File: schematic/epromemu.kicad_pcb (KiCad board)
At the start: 2 copper layers, 6 parts, among them J1 EPROM Connector, U1 Teensy4.1, U2 TXS0108EPW, U3 TXS0108EPW, U4 TXS0108EPW, U5 TXS0108EPW

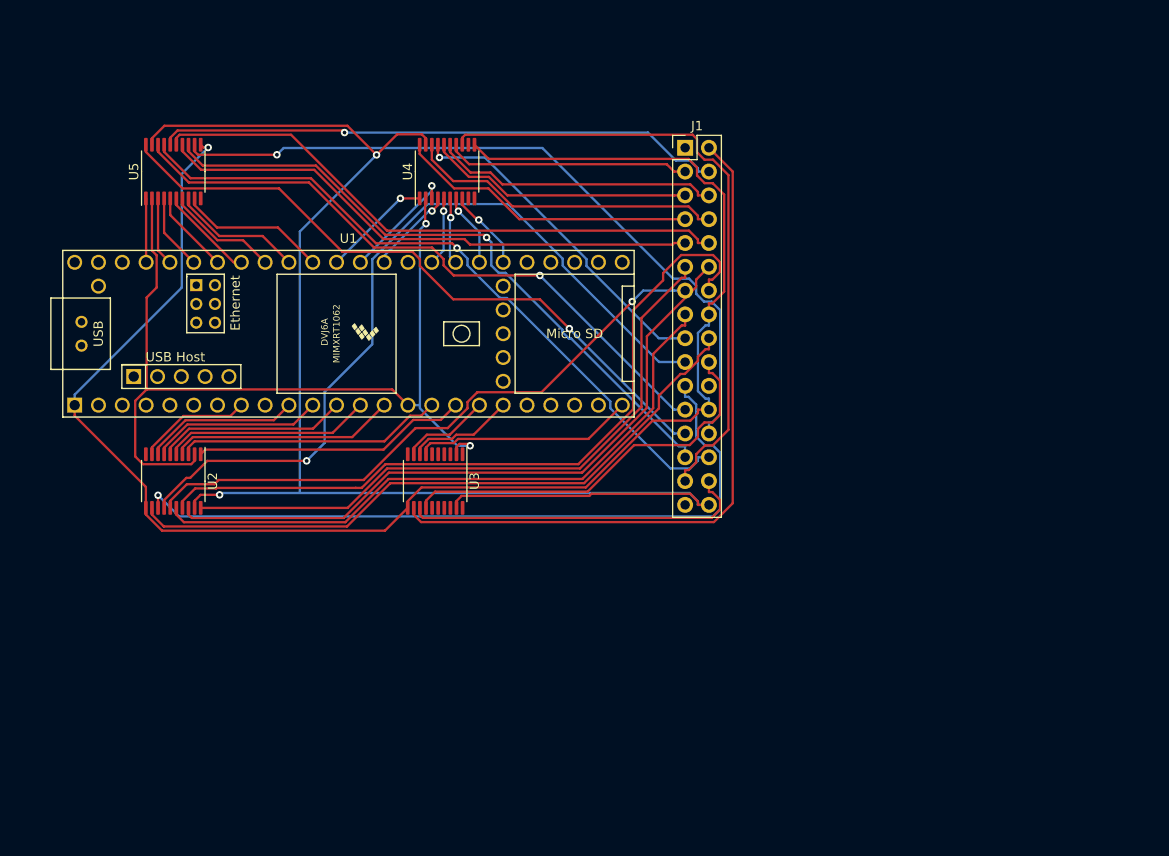
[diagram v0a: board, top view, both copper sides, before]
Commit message: updates
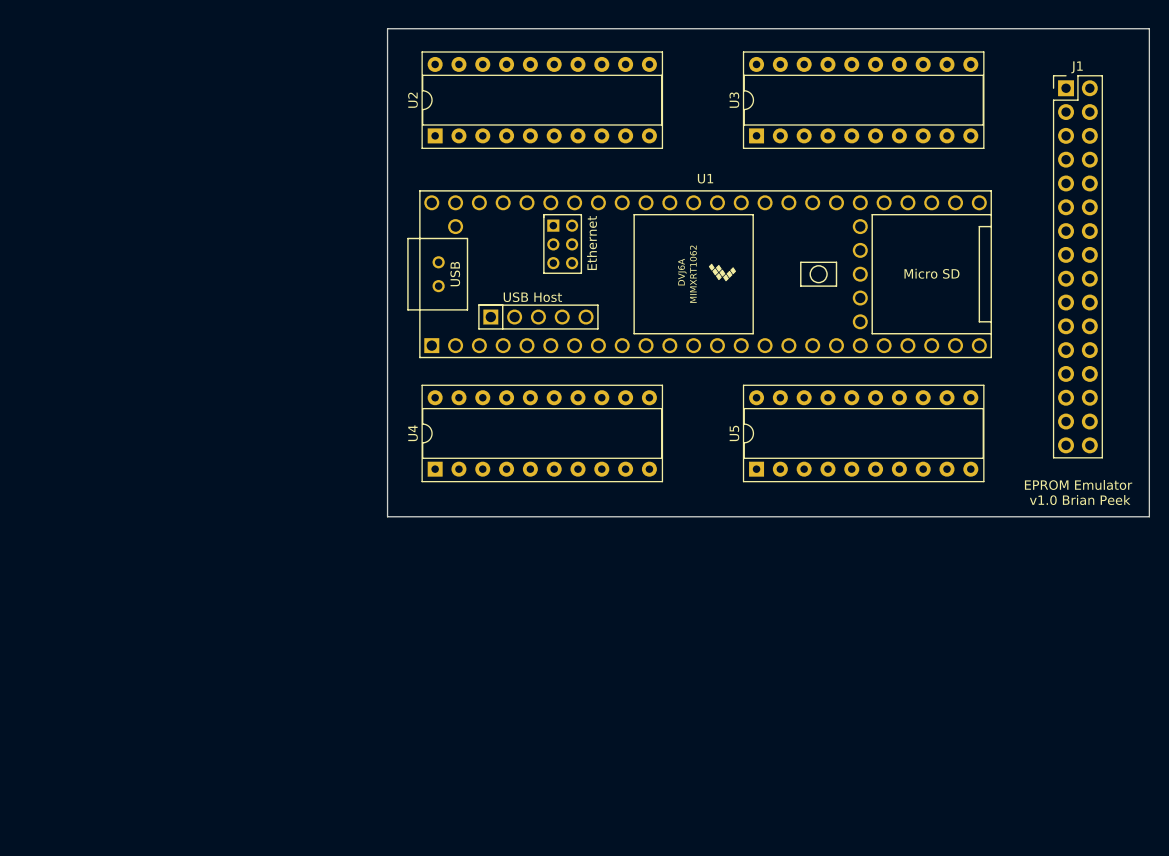
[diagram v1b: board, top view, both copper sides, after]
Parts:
- U2, U3, U4, U5: value TXS0108EPW -> 74HC245; footprint Package_SO:TSSOP-20_4.4x6.5mm_P0.65mm -> Package_DIP:DIP-20_W7.62mm_Socket
- moved U5 69.9 mm to (184.2, 85.1)
- moved U3 50.3 mm to (184.2, 49.5), turned to 90 degrees
- moved U2 46.2 mm to (149.9, 49.5), turned to 90 degrees
- moved J1 41.1 mm to (217.2, 44.5)
- moved U1 38.6 mm to (178.7, 64.3)
- moved U4 31.8 mm to (149.9, 85.1)
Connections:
- J1 pad 1: (no net) -> +5V
- J1 pad 22: (no net) -> CE_5V
- J1 pad 24: GND -> OE_5V
- J1 pad 31: (no net) -> PGM_5V
- U1 pad 25: (no net) -> PGM_3V3
- U1 pad 26: (no net) -> CE_3V3
- U2 pad 1: A1_3V3 -> GND
- U2 pad 10: (no net) -> GND
- U2 pad 11: GND -> D7_3V3
- U2 pad 12: D4_5V -> D6_3V3
- U2 pad 13: D7_5V -> D5_3V3
- U2 pad 14: D5_5V -> D4_3V3
- U2 pad 15: D0_5V -> D3_3V3
- U2 pad 16: D2_5V -> D2_3V3
- U2 pad 17: D1_5V -> D1_3V3
- U2 pad 18: A0_5V -> D0_3V3
- U2 pad 19: +5V -> OE_5V
- U2 pad 2: +3V3 -> D0_5V
- U2 pad 20: A1_5V -> +5V
- U2 pad 3: A0_3V3 -> D1_5V
- U2 pad 4: D1_3V3 -> D2_5V
- U2 pad 5: D2_3V3 -> D3_5V
- U2 pad 6: D0_3V3 -> D4_5V
- U2 pad 7: D5_3V3 -> D5_5V
- U2 pad 8: D7_3V3 -> D6_5V
- U2 pad 9: D4_3V3 -> D7_5V
- U3 pad 1: (no net) -> GND
- U3 pad 10: (no net) -> GND
- U3 pad 11: GND -> A7_5V
- U3 pad 12: A16_5V -> A6_5V
- U3 pad 13: A17_5V -> A5_5V
- U3 pad 14: D6_5V -> A4_5V
- U3 pad 15: (no net) -> A3_5V
- U3 pad 16: (no net) -> A2_5V
- U3 pad 17: (no net) -> A1_5V
- U3 pad 18: (no net) -> A0_5V
- U3 pad 19: +5V -> GND
- U3 pad 2: +3V3 -> A0_3V3
- U3 pad 20: (no net) -> +3V3
- U3 pad 3: (no net) -> A1_3V3
- U3 pad 4: (no net) -> A2_3V3
- U3 pad 5: (no net) -> A3_3V3
- U3 pad 6: (no net) -> A4_3V3
- U3 pad 7: D6_3V3 -> A5_3V3
- U3 pad 8: A17_3V3 -> A6_3V3
- U3 pad 9: A16_3V3 -> A7_3V3
- U4 pad 1: A5_3V3 -> GND
- U4 pad 10: (no net) -> GND
- U4 pad 11: GND -> A15_5V
- U4 pad 12: (no net) -> A14_5V
- U4 pad 13: A14_5V -> A13_5V
- U4 pad 14: A15_5V -> A12_5V
- U4 pad 15: A6_5V -> A11_5V
- U4 pad 16: A7_5V -> A10_5V
- U4 pad 17: D3_5V -> A9_5V
- U4 pad 18: A4_5V -> A8_5V
- U4 pad 19: +5V -> GND
- U4 pad 2: +3V3 -> A8_3V3
- U4 pad 20: A5_5V -> +3V3
- U4 pad 3: A4_3V3 -> A9_3V3
- U4 pad 4: D3_3V3 -> A10_3V3
- U4 pad 5: A7_3V3 -> A11_3V3
- U4 pad 6: A6_3V3 -> A12_3V3
- U4 pad 7: A15_3V3 -> A13_3V3
- U4 pad 9: (no net) -> A15_3V3
- U5 pad 1: A11_3V3 -> GND
- U5 pad 10: (no net) -> GND
- U5 pad 11: GND -> (no net)
- U5 pad 12: A9_5V -> (no net)
- U5 pad 13: A8_5V -> (no net)
- U5 pad 14: A3_5V -> PGM_5V
- U5 pad 15: A2_5V -> CE_5V
- U5 pad 16: A12_5V -> (no net)
- U5 pad 17: A13_5V -> A17_5V
- U5 pad 18: A10_5V -> A16_5V
- U5 pad 19: +5V -> GND
- U5 pad 2: +3V3 -> A16_3V3
- U5 pad 20: A11_5V -> +3V3
- U5 pad 3: A10_3V3 -> A17_3V3
- U5 pad 4: A13_3V3 -> (no net)
- U5 pad 5: A12_3V3 -> CE_3V3
- U5 pad 6: A2_3V3 -> PGM_3V3
- U5 pad 7: A3_3V3 -> (no net)
- U5 pad 8: A8_3V3 -> (no net)
- U5 pad 9: A9_3V3 -> (no net)
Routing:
- net GND: track 170.5 -> 0.00 mm, vias 1 -> 0
- net +5V: track 158.4 -> 0.00 mm, vias 2 -> 0
- net +3V3: track 98.3 -> 0.00 mm, vias 2 -> 0
- net D5_5V: track 85.4 -> 0.00 mm, vias 1 -> 0
- net D1_5V: track 79.7 -> 0.00 mm
- net A9_5V: track 78.8 -> 0.00 mm, vias 1 -> 0
- net D7_5V: track 78.0 -> 0.00 mm, vias 1 -> 0
- net A16_5V: track 74.9 -> 0.00 mm
- net A13_5V: track 74.4 -> 0.00 mm, vias 1 -> 0
- net A0_5V: track 72.4 -> 0.00 mm
- net A11_5V: track 71.2 -> 0.00 mm, vias 1 -> 0
- net D4_5V: track 70.7 -> 0.00 mm
- net A8_5V: track 69.5 -> 0.00 mm, vias 1 -> 0
- net A10_5V: track 68.8 -> 0.00 mm, vias 1 -> 0
- net D2_5V: track 68.6 -> 0.00 mm
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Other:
- board outline added: 81.3 x 52.1 mm
- board text added: "EPROM Emulator v1.0 Brian Peek"

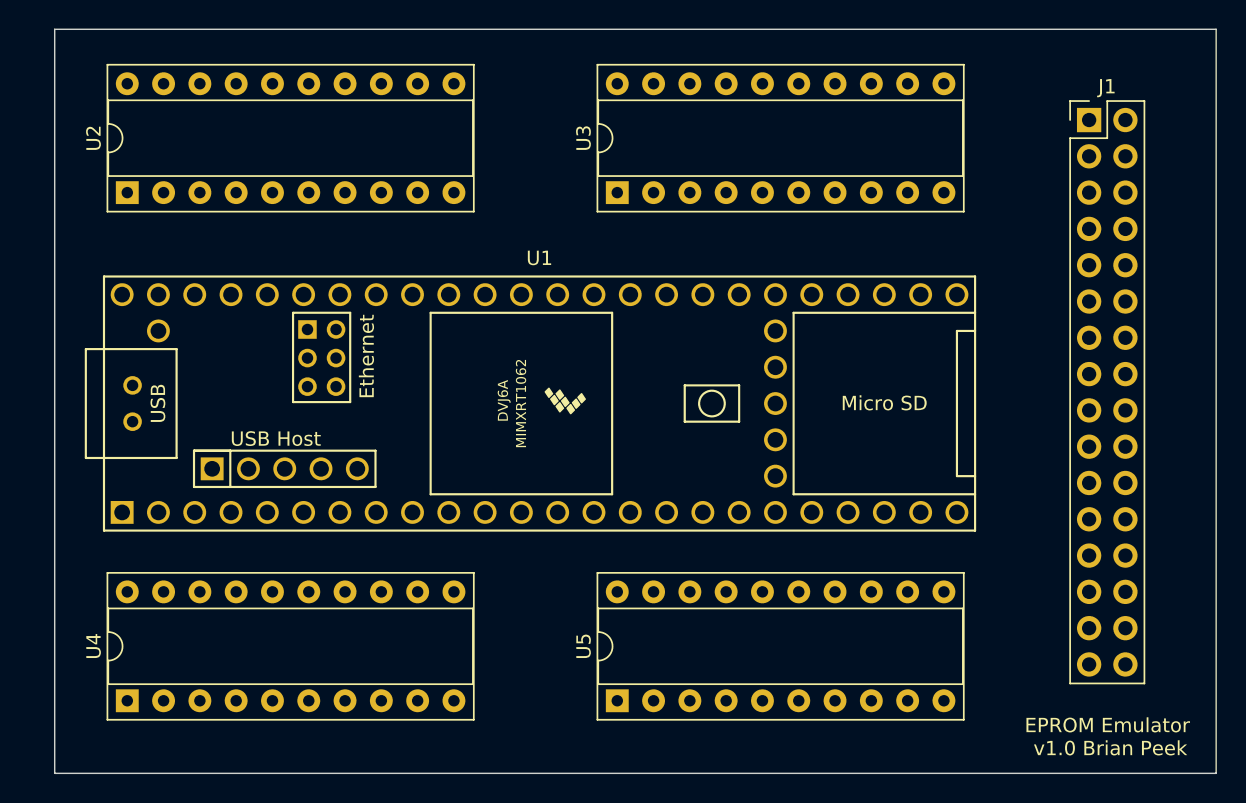
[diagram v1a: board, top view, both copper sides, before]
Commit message: update
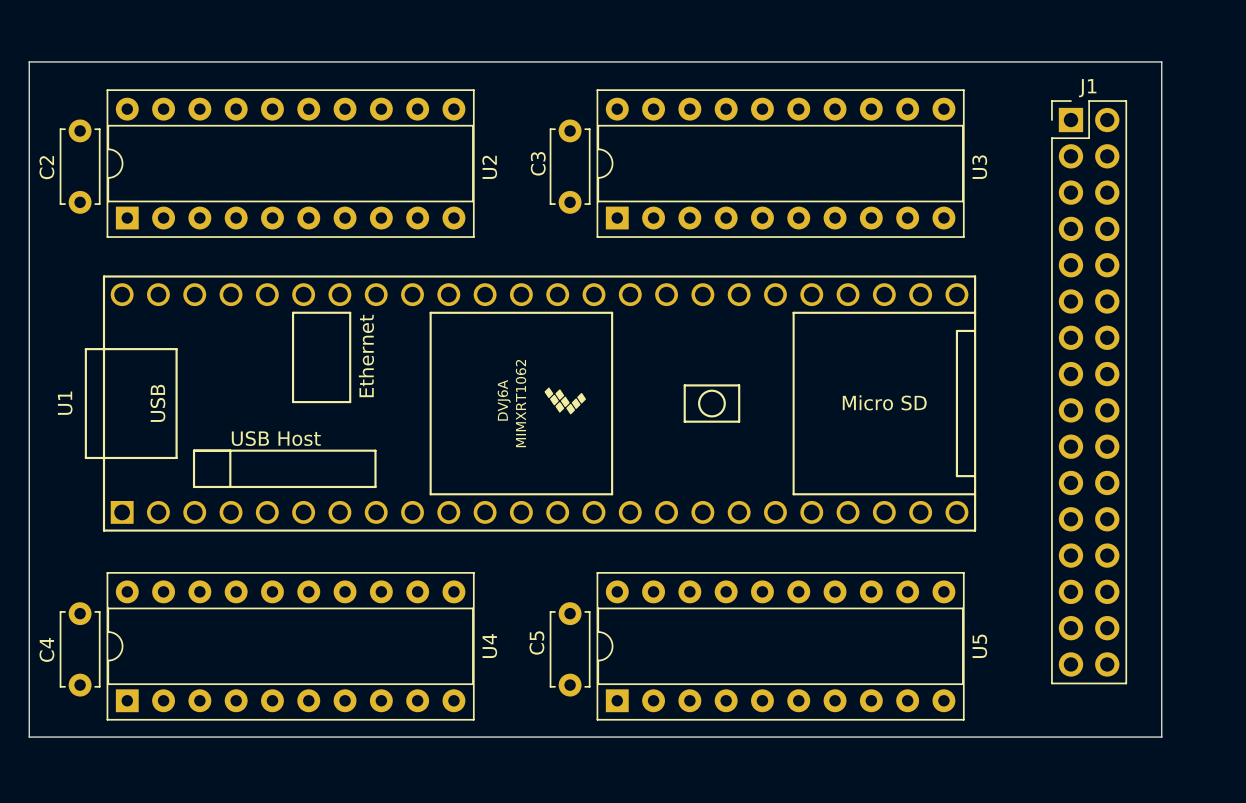
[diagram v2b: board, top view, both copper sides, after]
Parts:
- added C2: 0.1uf, Capacitor_THT:C_Disc_D5.0mm_W2.5mm_P5.00mm, F.Cu at (146.6, 45.2)
- added C3: 0.1uf, Capacitor_THT:C_Disc_D5.0mm_W2.5mm_P5.00mm, F.Cu at (180.8, 45.2)
- added C4: 0.1uf, Capacitor_THT:C_Disc_D5.0mm_W2.5mm_P5.00mm, F.Cu at (146.6, 79.0)
- added C5: 0.1uf, Capacitor_THT:C_Disc_D5.0mm_W2.5mm_P5.00mm, F.Cu at (180.8, 79.0)
- moved U2 1.78 mm to (149.9, 51.3)
- moved U3 1.78 mm to (184.2, 51.3)
- moved J1 1.27 mm to (215.9, 44.5)
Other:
- board size 81.3 x 52.1 mm -> 79.2 x 47.2 mm
- board text removed: "EPROM Emulator v1.0 Brian Peek"

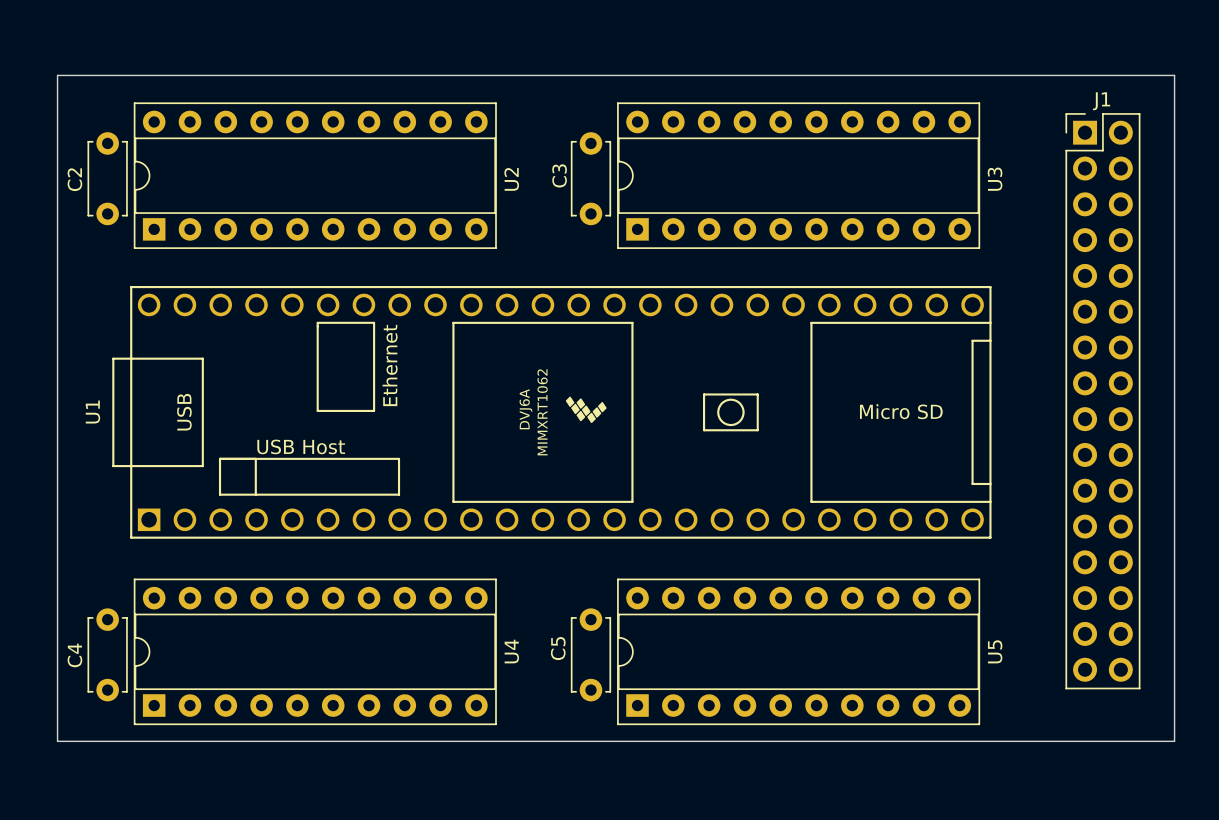
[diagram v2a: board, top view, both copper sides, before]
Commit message: updates'
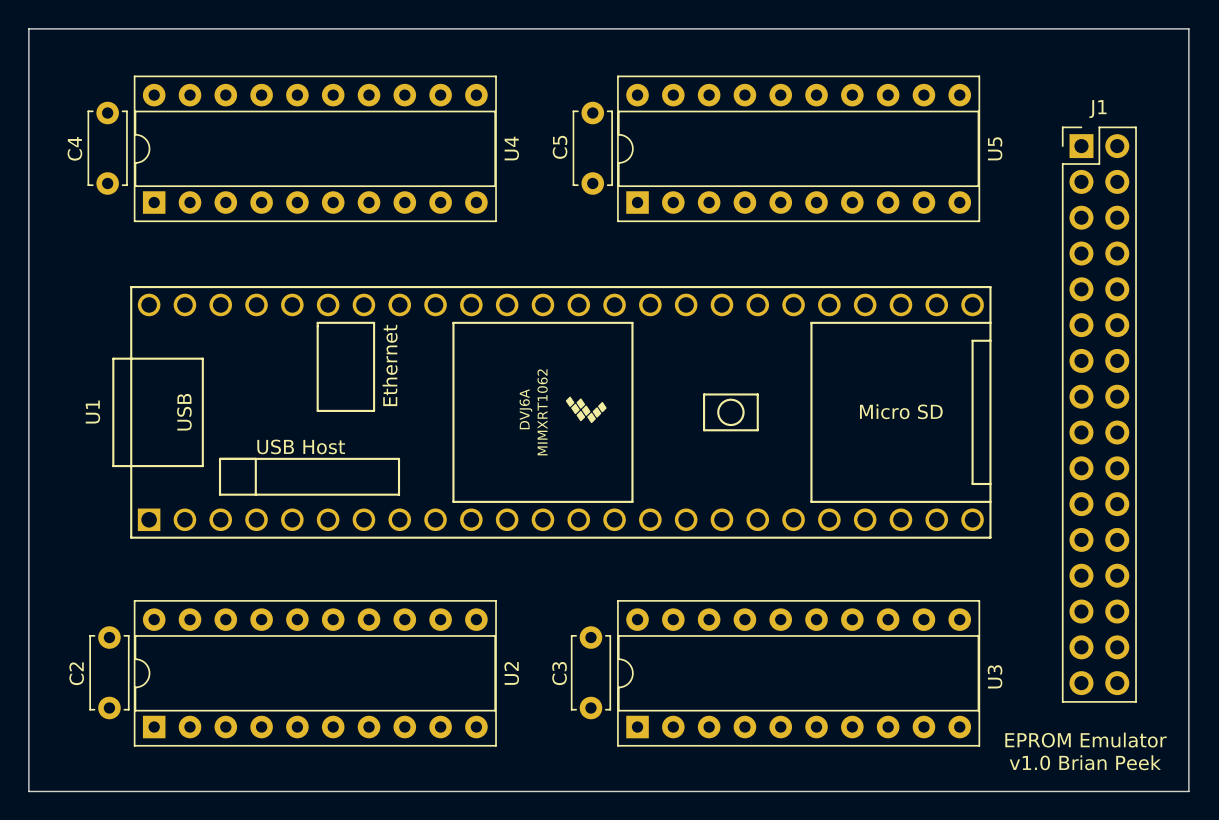
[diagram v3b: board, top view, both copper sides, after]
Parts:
- moved C5 35.9 mm to (181.0, 43.1)
- moved C4 35.9 mm to (146.6, 43.1)
- moved U4 35.7 mm to (149.9, 49.4)
- moved U5 35.7 mm to (184.2, 49.4)
- moved U2 35.3 mm to (149.9, 86.6)
- moved U3 35.3 mm to (184.2, 86.6)
- moved C2 35.1 mm to (146.7, 80.3)
- moved C3 35.1 mm to (180.8, 80.3)
- moved J1 0.98 mm to (215.6, 45.4)
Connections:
- U2 pad 11: D7_3V3 -> D3_3V3
- U2 pad 13: D5_3V3 -> D1_3V3
- U2 pad 14: D4_3V3 -> D2_3V3
- U2 pad 15: D3_3V3 -> D0_3V3
- U2 pad 16: D2_3V3 -> D5_3V3
- U2 pad 17: D1_3V3 -> D7_3V3
- U2 pad 18: D0_3V3 -> D4_3V3
- U2 pad 2: D0_5V -> D4_5V
- U2 pad 3: D1_5V -> D7_5V
- U2 pad 4: D2_5V -> D5_5V
- U2 pad 5: D3_5V -> D0_5V
- U2 pad 6: D4_5V -> D2_5V
- U2 pad 7: D5_5V -> D1_5V
- U2 pad 9: D7_5V -> D3_5V
- U3 pad 11: A7_5V -> (no net)
- U3 pad 12: A6_5V -> (no net)
- U3 pad 13: A5_5V -> (no net)
- U3 pad 14: A4_5V -> (no net)
- U3 pad 15: A3_5V -> A17_3V3
- U3 pad 16: A2_5V -> A16_3V3
- U3 pad 17: A1_5V -> A1_3V3
- U3 pad 18: A0_5V -> A0_3V3
- U3 pad 2: A0_3V3 -> A0_5V
- U3 pad 3: A1_3V3 -> A1_5V
- U3 pad 4: A2_3V3 -> A16_5V
- U3 pad 5: A3_3V3 -> A17_5V
- U3 pad 6: A4_3V3 -> (no net)
- U3 pad 7: A5_3V3 -> (no net)
- U3 pad 8: A6_3V3 -> (no net)
- U3 pad 9: A7_3V3 -> (no net)
- U4 pad 1: GND -> +3V3
- U4 pad 11: A15_5V -> A9_5V
- U4 pad 12: A14_5V -> A8_5V
- U4 pad 13: A13_5V -> A3_5V
- U4 pad 14: A12_5V -> A2_5V
- U4 pad 15: A11_5V -> A12_5V
- U4 pad 16: A10_5V -> A13_5V
- U4 pad 17: A9_5V -> A10_5V
- U4 pad 18: A8_5V -> A11_5V
- U4 pad 2: A8_3V3 -> A11_3V3
- U4 pad 3: A9_3V3 -> A10_3V3
- U4 pad 4: A10_3V3 -> A13_3V3
- U4 pad 5: A11_3V3 -> A12_3V3
- U4 pad 6: A12_3V3 -> A2_3V3
- U4 pad 7: A13_3V3 -> A3_3V3
- U4 pad 8: A14_3V3 -> A8_3V3
- U4 pad 9: A15_3V3 -> A9_3V3
- U5 pad 1: GND -> +3V3
- U5 pad 11: (no net) -> PGM_5V
- U5 pad 12: (no net) -> CE_5V
- U5 pad 13: (no net) -> A15_5V
- U5 pad 14: PGM_5V -> A14_5V
- U5 pad 15: CE_5V -> A6_5V
- U5 pad 16: (no net) -> A7_5V
- U5 pad 17: A17_5V -> A4_5V
- U5 pad 18: A16_5V -> A5_5V
- U5 pad 2: A16_3V3 -> A5_3V3
- U5 pad 3: A17_3V3 -> A4_3V3
- U5 pad 4: (no net) -> A7_3V3
- U5 pad 5: CE_3V3 -> A6_3V3
- U5 pad 6: PGM_3V3 -> A15_3V3
- U5 pad 7: (no net) -> A14_3V3
- U5 pad 8: (no net) -> CE_3V3
- U5 pad 9: (no net) -> PGM_3V3
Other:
- board size 79.2 x 47.2 mm -> 82.3 x 54.1 mm
- board text added: "EPROM Emulator v1.0 Brian Peek"
